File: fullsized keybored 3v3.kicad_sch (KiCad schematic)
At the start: 51 parts, among them IC1 W25Q16JVUXIQ, J1 USB_C_Receptacle_USB2.0, J10 Conn_01x01, J2 Conn_01x06, J3 Conn_01x01, J4 Conn_01x01, J9 Conn_01x01, SW1 boot, U1 RP2040, U2 USBLC6-2SC6, U3 XC6206PxxxMR-Regulator_Linear, Y1 12MHz

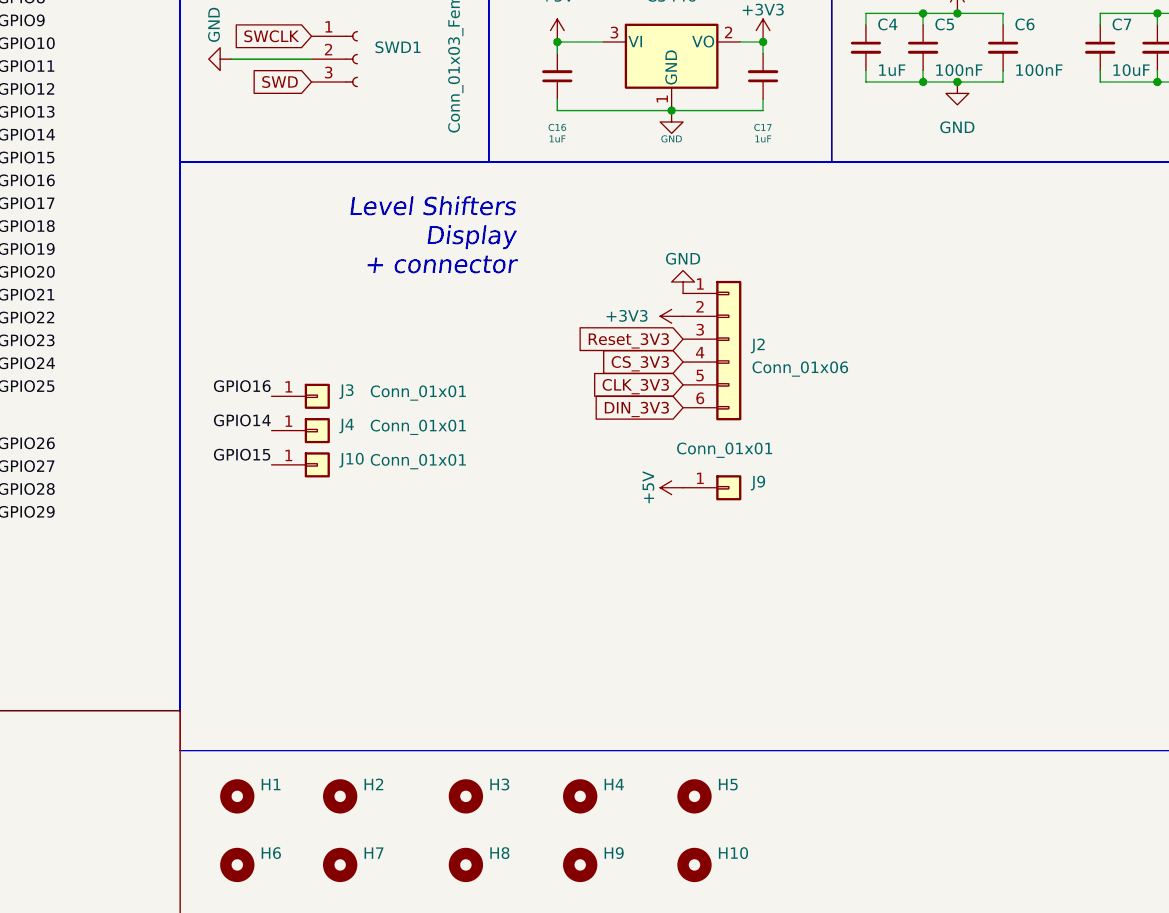
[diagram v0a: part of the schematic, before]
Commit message: production files ready
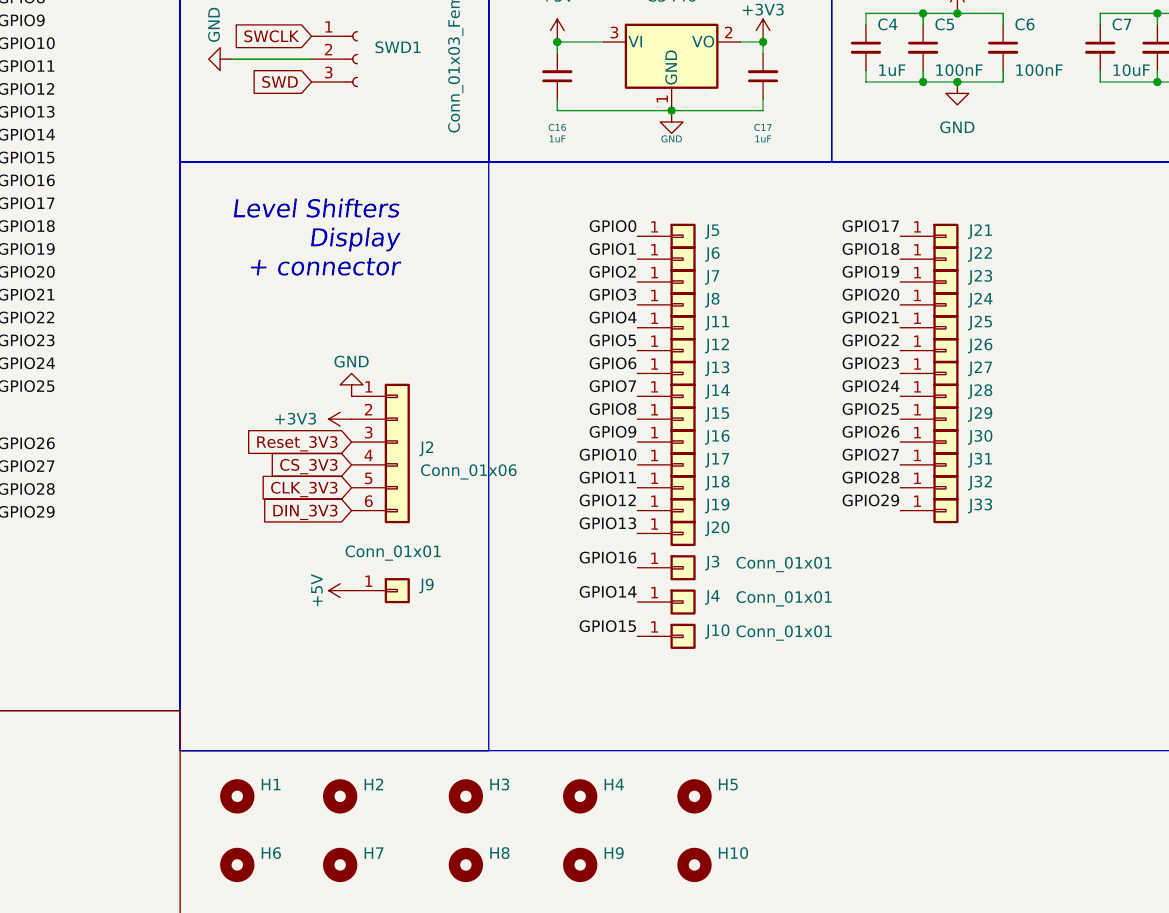
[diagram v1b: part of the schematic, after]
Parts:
- added J11, J12, J13, J14, J15, J16, J17, J18, J19, J20, J21, J22, J23, J24, J25, J26, J27, J28, J29, J30, J31, J32, J33, J5, J6, J7, J8: Conn_01x01, TestPoint:TestPoint_THTPad_D1.5mm_Drill0.7mm, symbol Connector_Generic:Conn_01x01
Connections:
- net CLK_3V3: now also J7.1 (Pin_1)
- net COL0: now also J33.1 (Pin_1)
- net COL1: now also J32.1 (Pin_1)
- net COL10: now also J11.1 (Pin_1)
- net COL2: now also J31.1 (Pin_1)
- net COL3: now also J30.1 (Pin_1)
- net COL4: now also J29.1 (Pin_1)
- net COL5: now also J28.1 (Pin_1)
- net COL6: now also J27.1 (Pin_1)
- net COL7: now also J14.1 (Pin_1)
- net COL8: now also J13.1 (Pin_1)
- net COL9: now also J12.1 (Pin_1)
- net CS_3V3: now also J6.1 (Pin_1)
- net DIN_3V3: now also J8.1 (Pin_1)
- net ROW0: now also J21.1 (Pin_1)
- net ROW1: now also J22.1 (Pin_1)
- net ROW10: now also J16.1 (Pin_1)
- net ROW11: now also J15.1 (Pin_1)
- net ROW2: now also J23.1 (Pin_1)
- net ROW3: now also J24.1 (Pin_1)
- net ROW4: now also J25.1 (Pin_1)
- net ROW5: now also J26.1 (Pin_1)
- net ROW6: now also J20.1 (Pin_1)
- net ROW7: now also J19.1 (Pin_1)
- net ROW8: now also J18.1 (Pin_1)
- net ROW9: now also J17.1 (Pin_1)
- net Reset_3V3: now also J5.1 (Pin_1)
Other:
- moved on the sheet: J10, J2, J3, J4, J9
